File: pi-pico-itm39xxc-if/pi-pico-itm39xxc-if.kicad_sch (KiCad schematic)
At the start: 15 parts

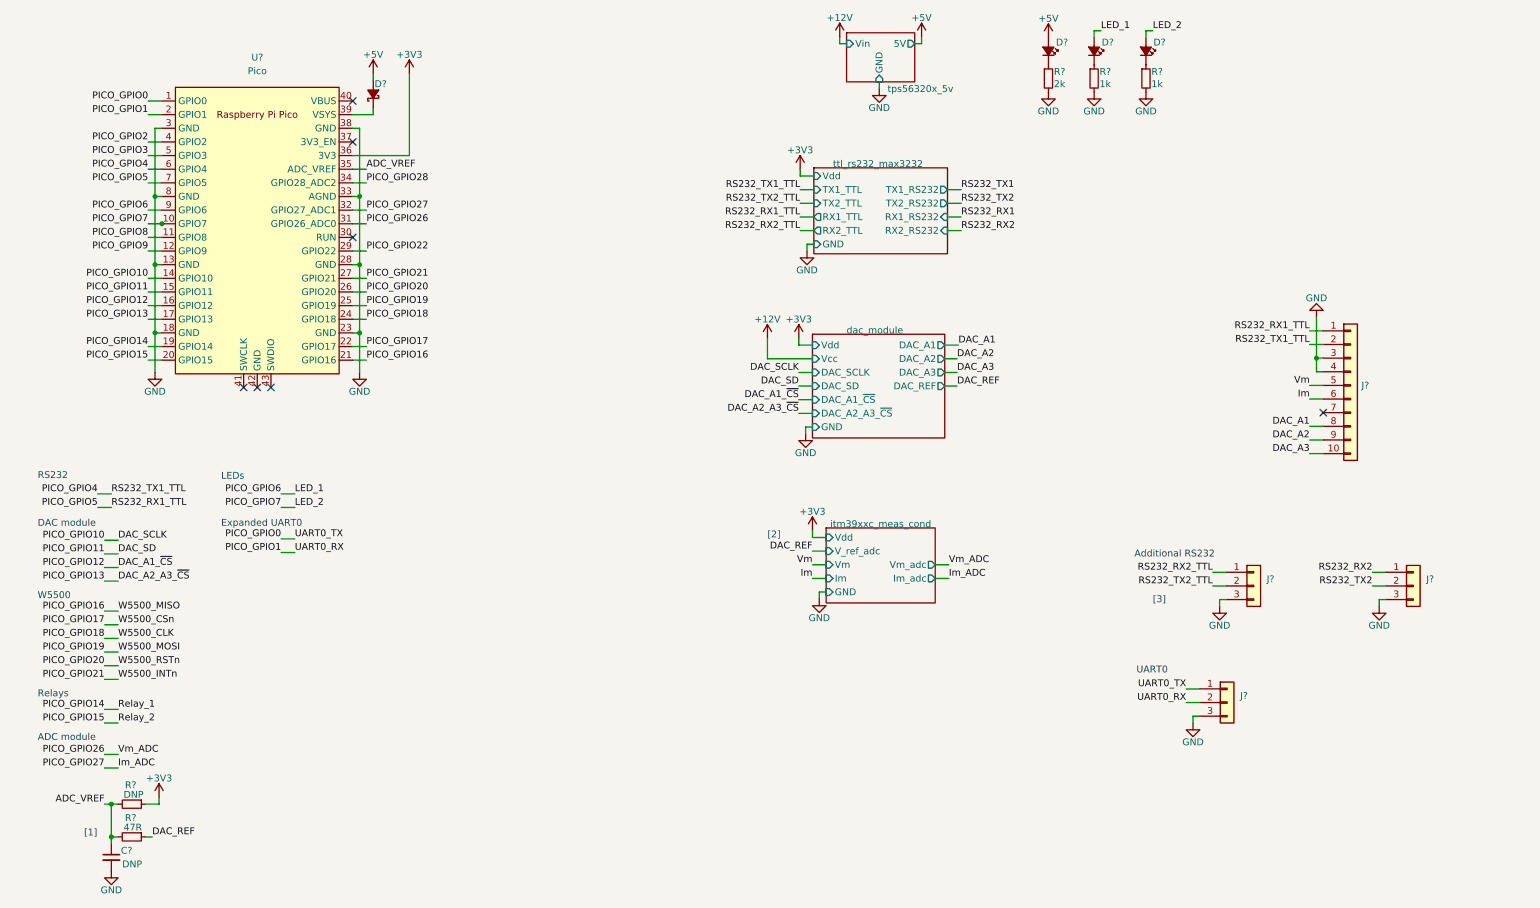
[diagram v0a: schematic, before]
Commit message: Finishing schematics of pico itm if
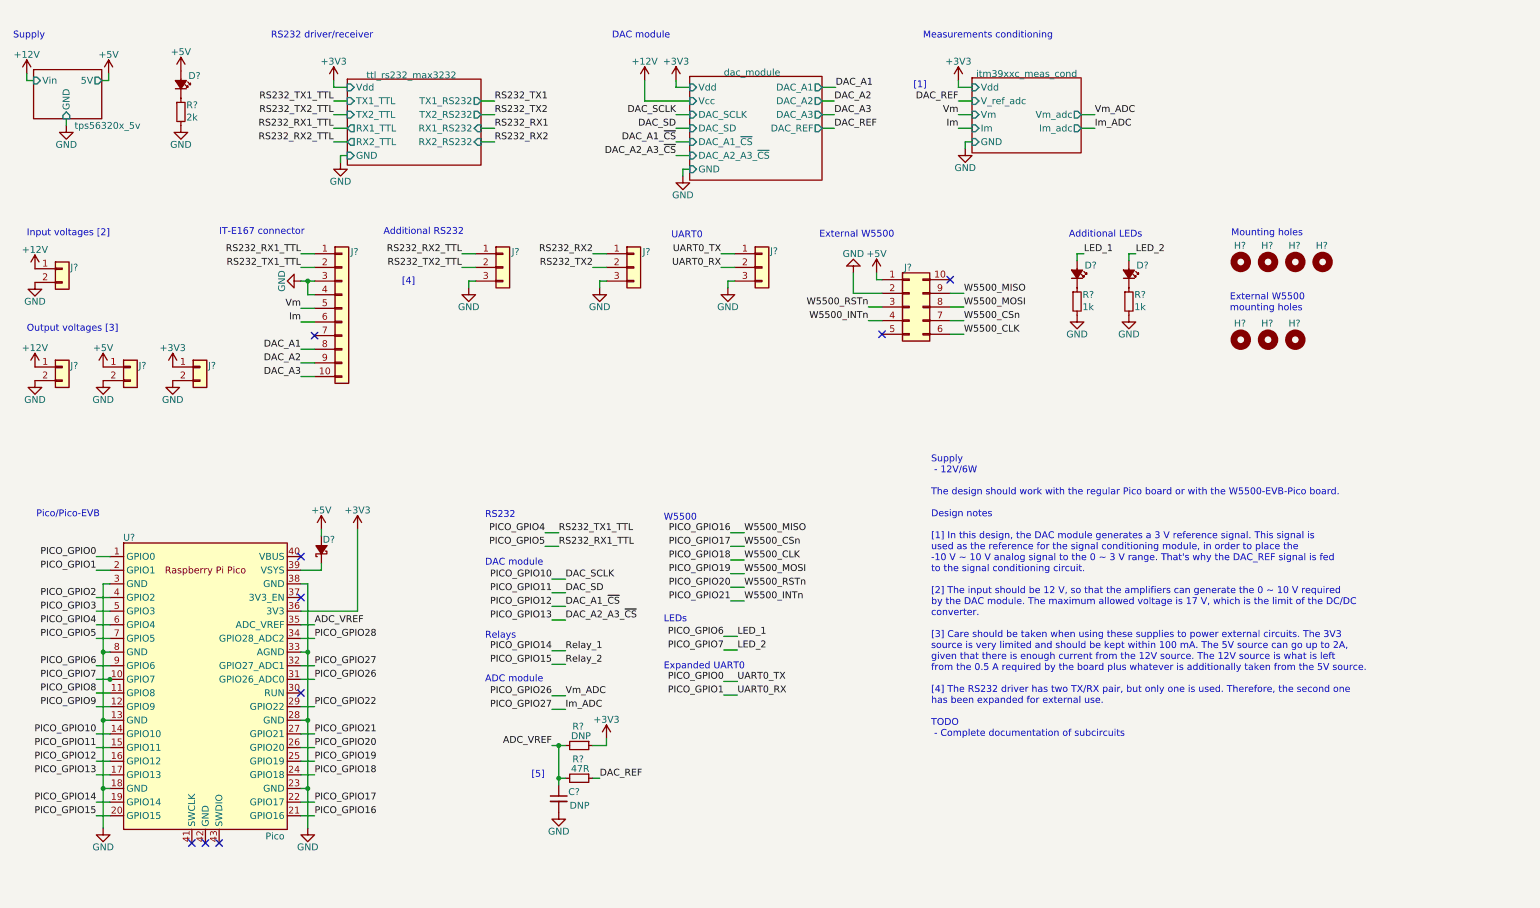
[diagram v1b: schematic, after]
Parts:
- added H? (x7): MountingHole, MountingHole:MountingHole_3.2mm_M3, symbol Mechanical:MountingHole
- added J? (x4): Conn_01x02, TerminalBlock_Phoenix:TerminalBlock_Phoenix_MKDS-1,5-2-5.08_1x02_P5.08mm_Horizontal, symbol Connector_Generic:Conn_01x02
- added J?: Conn_02x05_Counter_Clockwise, symbol Connector_Generic:Conn_02x05_Counter_Clockwise
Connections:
- net +12V: now also J?.1 (Pin_1), J?.1 (Pin_1)
- net +3V3: now also J?.1 (Pin_1)
- net +5V: now also J?.1 (Pin_1), J?.1 (Pin_1)
- net GND: now also J?.2 (Pin_2), J?.2 (Pin_2), J?.2 (Pin_2), J?.2 (Pin_2), J?.2 (Pin_2)
- net PICO_GPIO16: now also J?.9 (Pin_9)
- net PICO_GPIO17: now also J?.7 (Pin_7)
- net PICO_GPIO18: now also J?.6 (Pin_6)
- net PICO_GPIO19: now also J?.8 (Pin_8)
- net PICO_GPIO20: now also J?.3 (Pin_3)
- net PICO_GPIO21: now also J?.4 (Pin_4)
- no-connect marks 7 -> 9
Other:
- note added: "Additional LEDs"
- note added: "External W5500"
- note added: "External W5500 mounting holes"
- note added: "IT-E167 connector"
- note added: "Input voltages [2]"
- note added: "Measurements conditioning"
- note added: "Mounting holes"
- note added: "Output voltages [3]"
- note added: "Pico/Pico-EVB"
- note added: "RS232 driver/receiver"
- note added: "Supply"
- note added: "Supply - 12V/6W The design should work with the regular Pico board or with the W5500-EVB-Pico board. Design notes [1] In this design, the DAC module generates a 3 V reference signal. This signal is used as the reference for the signal conditioning module, in order to place the -10 V ~ 10 V analog signal to the 0 ~ 3 V range. That's why the DAC_REF signal is fed to the signal conditioning circuit.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"
- note added: "[4]"
- note added: "[5]"
- note removed: "[2]"
- note removed: "[3]"
- moved on the sheet: C?, D?, J?, R?, U?
